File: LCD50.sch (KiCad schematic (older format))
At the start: 36 parts, among them Q10 IRLML2502, Q8 IRLML2502, Q9 IRLML2502, U8 xc7z020clg400

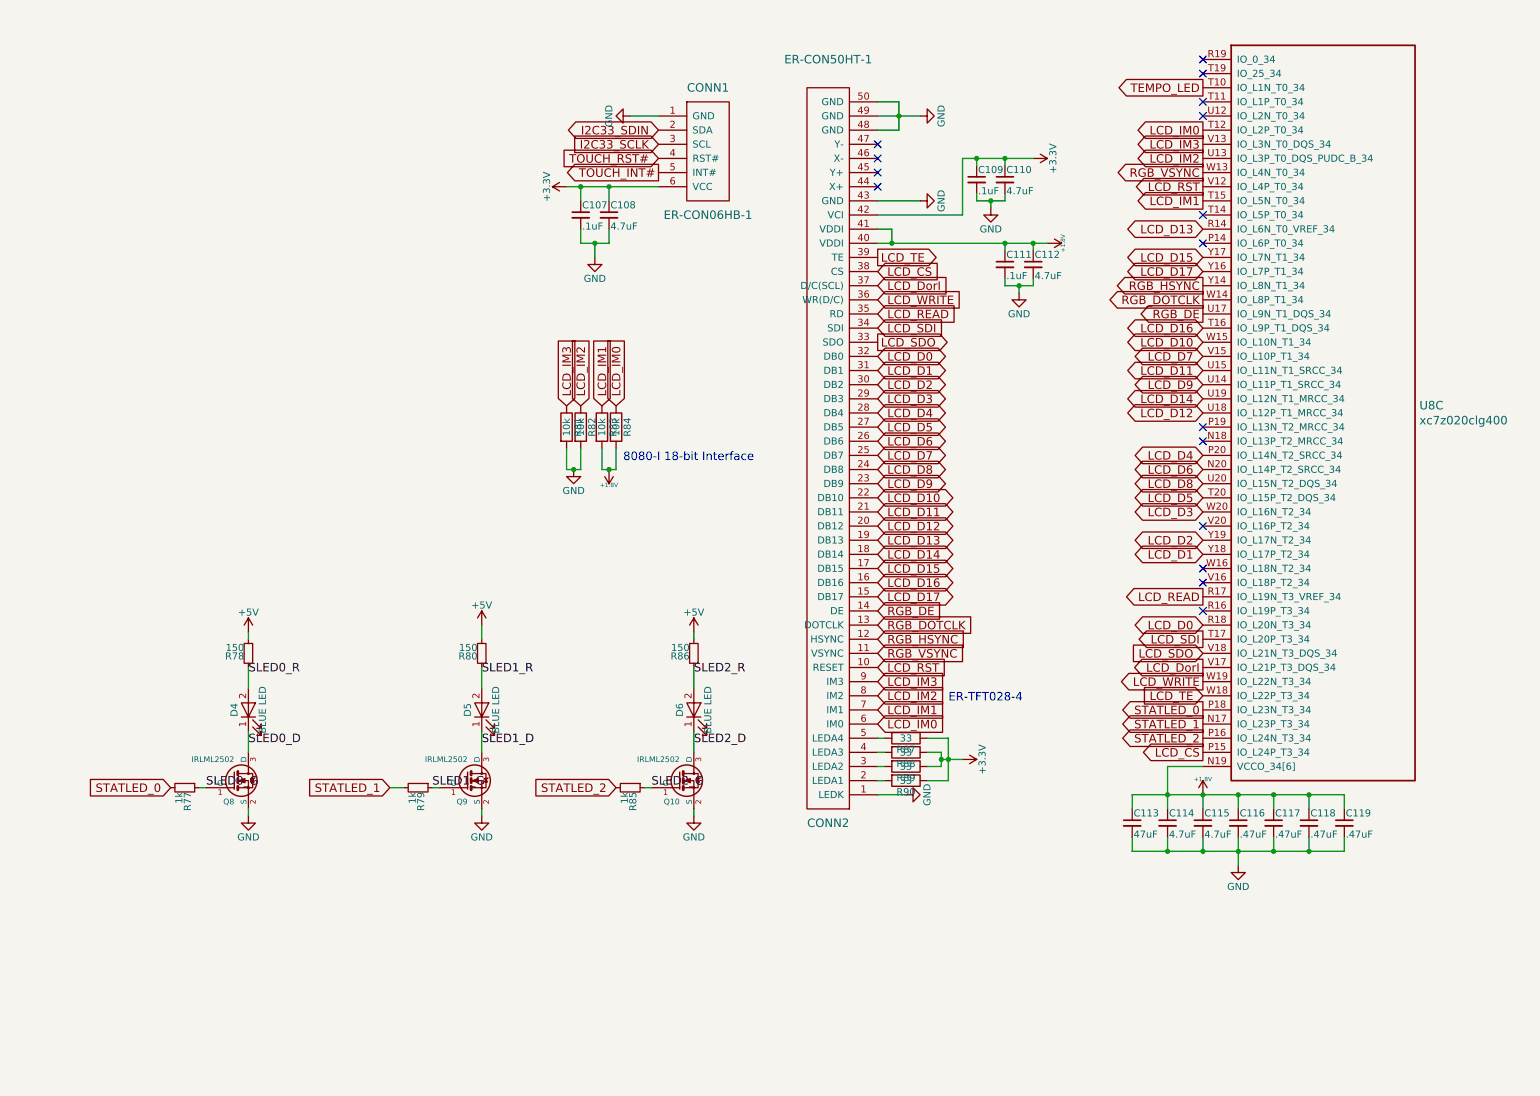
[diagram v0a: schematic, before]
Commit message: random updates
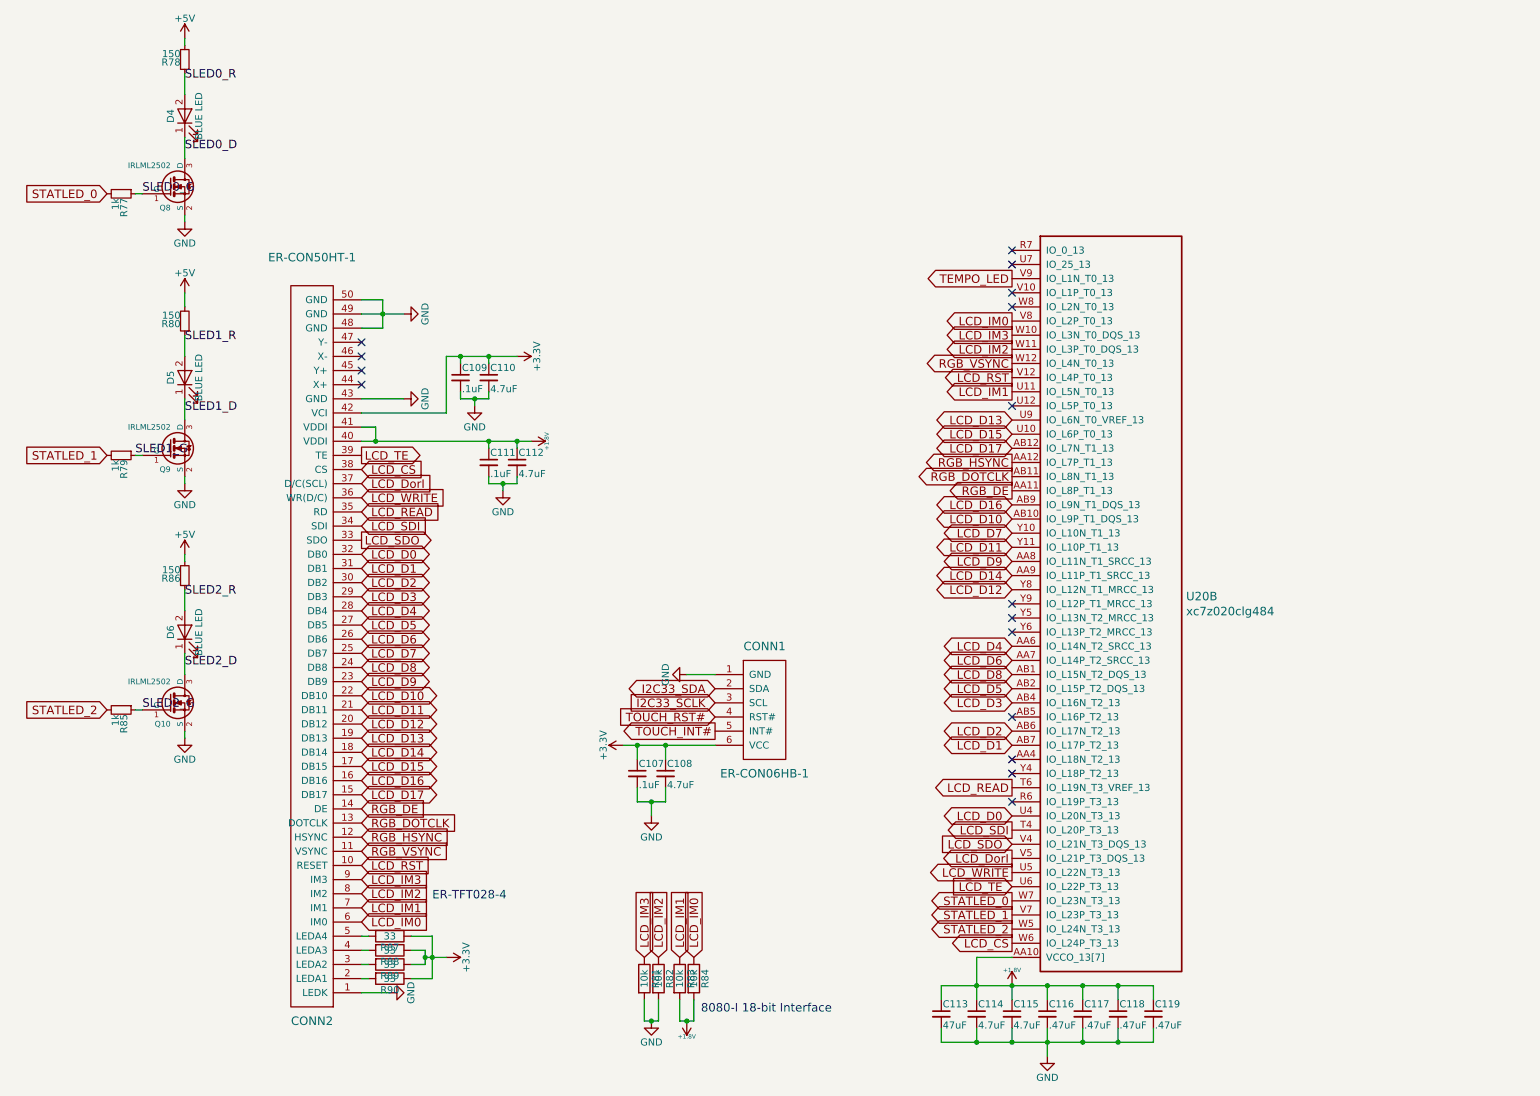
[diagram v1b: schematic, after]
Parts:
- removed U8: xc7z020clg400, DFTcustom:BGA400_0.8p_17mmx17mm, symbol DFTBoard-rescue:xc7z020clg400-
- added U20: xc7z020clg484, DFTcustom:BGA-484_19.0x19.0mm_Layout22x22_P0.80mm_dia0.40mm, symbol xilinx7:xc7z020clg484
- C107, C108, C109, C110, C111, C112, C114, C115, C116, C117, C118, C119: footprint Capacitor_SMD:C_0603_1608Metric -> Capacitor_SMD:C_0402_1005Metric
- D4, D5, D6: footprint LEDs:LED_0603 -> Capacitor_SMD:C_0603_1608Metric
- R77, R78, R79, R80, R81, R82, R83, R84, R85, R86, R87, R88, R89, R90: footprint Resistors_SMD:R_0402 -> Resistor_SMD:R_0402_1005Metric
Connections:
- net +1V8: now also U20.AA10 (VCCO_13[7]), U20.AB3 (VCCO_13[7]), U20.T5 (VCCO_13[7]), U20.U8 (VCCO_13[7]), U20.V11 (VCCO_13[7]), U20.W4 (VCCO_13[7]), U20.Y7 (VCCO_13[7])
- net LCD_CS: now also U20.W6 (IO_L24P_T3_13)
- net LCD_D0: now also U20.U4 (IO_L20N_T3_13)
- net LCD_D1: now also U20.AB7 (IO_L17P_T2_13)
- net LCD_D10: now also U20.AB10 (IO_L9P_T1_DQS_13)
- net LCD_D11: now also U20.Y11 (IO_L10P_T1_13)
- net LCD_D12: now also U20.Y8 (IO_L12N_T1_MRCC_13)
- net LCD_D13: now also U20.U9 (IO_L6N_T0_VREF_13)
- net LCD_D14: now also U20.AA9 (IO_L11P_T1_SRCC_13)
- net LCD_D15: now also U20.U10 (IO_L6P_T0_13)
- net LCD_D16: now also U20.AB9 (IO_L9N_T1_DQS_13)
- net LCD_D17: now also U20.AB12 (IO_L7N_T1_13)
- net LCD_D2: now also U20.AB6 (IO_L17N_T2_13)
- net LCD_D3: now also U20.AB4 (IO_L16N_T2_13)
- net LCD_D4: now also U20.AA6 (IO_L14N_T2_SRCC_13)
- net LCD_D5: now also U20.AB2 (IO_L15P_T2_DQS_13)
- net LCD_D6: now also U20.AA7 (IO_L14P_T2_SRCC_13)
- net LCD_D7: now also U20.Y10 (IO_L10N_T1_13)
- net LCD_D8: now also U20.AB1 (IO_L15N_T2_DQS_13)
- net LCD_D9: now also U20.AA8 (IO_L11N_T1_SRCC_13)
- net LCD_DorI: now also U20.V5 (IO_L21P_T3_DQS_13)
- net LCD_IM0: now also U20.V8 (IO_L2P_T0_13)
- net LCD_IM1: now also U20.U11 (IO_L5N_T0_13)
- net LCD_IM2: now also U20.W11 (IO_L3P_T0_DQS_13)
- net LCD_IM3: now also U20.W10 (IO_L3N_T0_DQS_13)
- net LCD_READ: now also U20.T6 (IO_L19N_T3_VREF_13)
- net LCD_RST: now also U20.V12 (IO_L4P_T0_13)
- net LCD_SDI: now also U20.T4 (IO_L20P_T3_13)
- net LCD_SDO: now also U20.V4 (IO_L21N_T3_DQS_13)
- net LCD_TE: now also U20.U6 (IO_L22P_T3_13)
- net LCD_WRITE: now also U20.U5 (IO_L22N_T3_13)
- net RGB_DE: now also U20.AA11 (IO_L8P_T1_13)
- net RGB_DOTCLK: now also U20.AB11 (IO_L8N_T1_13)
- net RGB_HSYNC: now also U20.AA12 (IO_L7P_T1_13)
- net RGB_VSYNC: now also U20.W12 (IO_L4N_T0_13)
- net STATLED_0: now also U20.W7 (IO_L23N_T3_13)
- net STATLED_1: now also U20.V7 (IO_L23P_T3_13)
- net STATLED_2: now also U20.W5 (IO_L24N_T3_13)
- net TEMPO_LED: now also U20.V9 (IO_L1N_T0_13)
- net I2C33_SDIN renamed I2C33_SDA
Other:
- moved on the sheet: C107, C108, C109, C110, C111, C112, C113, C114, C115, C116, C117, C118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
